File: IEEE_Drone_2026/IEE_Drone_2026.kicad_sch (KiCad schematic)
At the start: 31 parts, among them IC1 TPSM84209RKHT, IC2 TPSM84209RKHT, J1 ESC, J10 M2, J11 Conn_01x02_Socket, J2 M4 Mounting, J3 M4 Mounting, J4 M4 Mounting, J5 M4 Mounting, J6 Pixy2, J7 M2, J8 M2, J9 M2, Q1 2N2222, U1 MS560702BA03-50

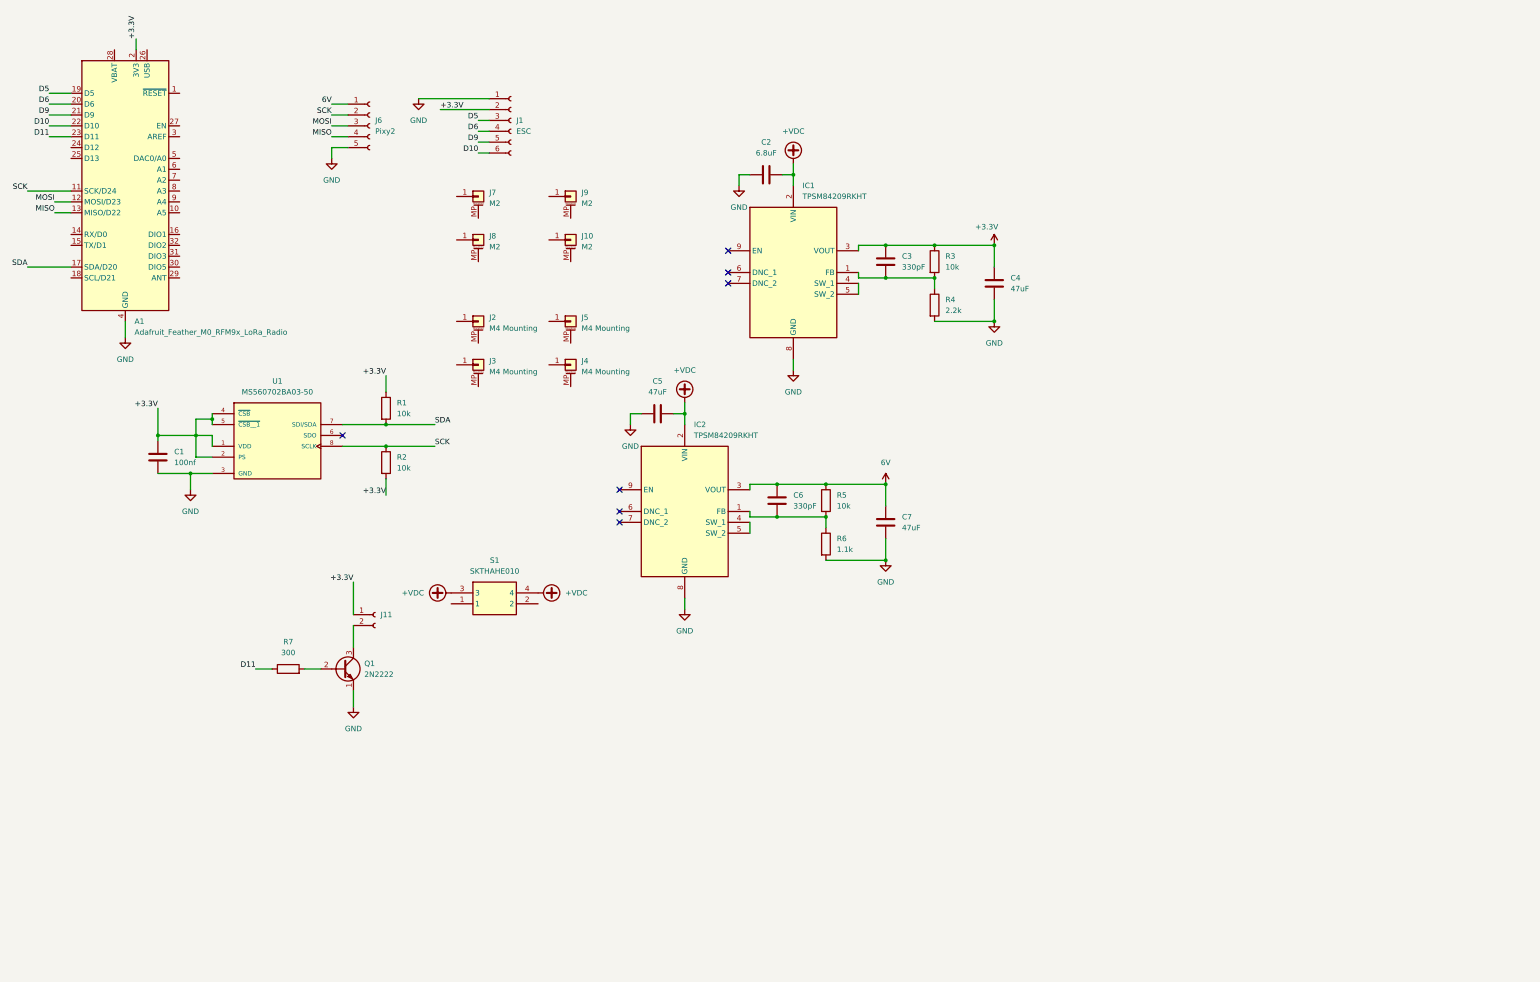
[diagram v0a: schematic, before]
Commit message: update sch last time before redesign
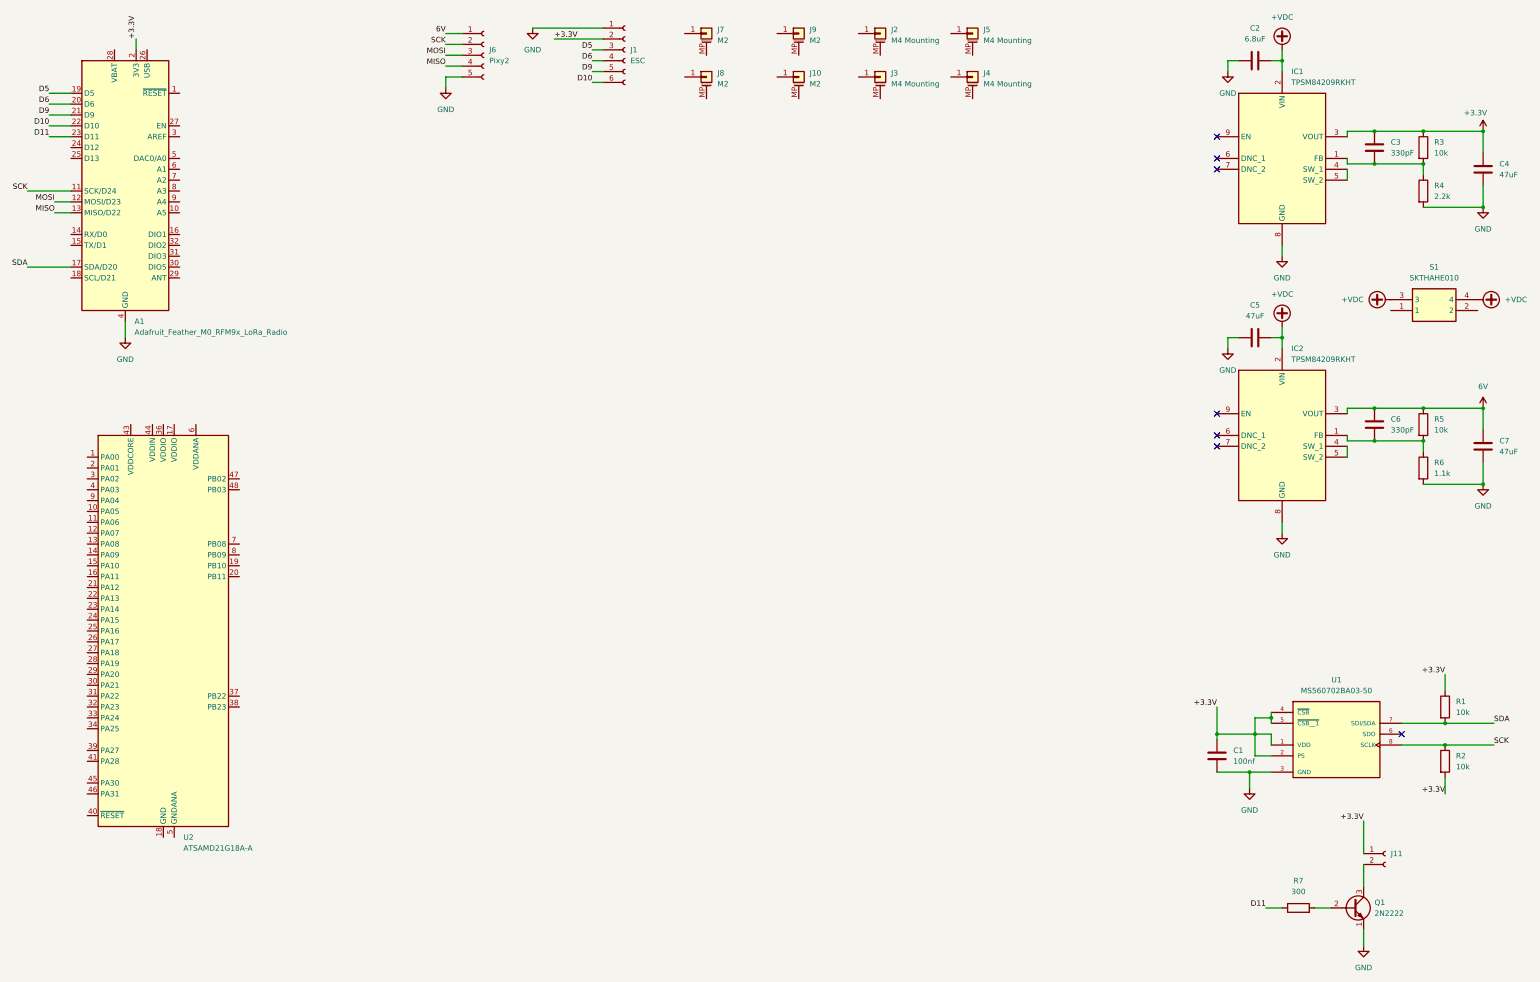
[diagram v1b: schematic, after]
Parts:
- added U2: ATSAMD21G18A-A, Package_QFP:TQFP-48_7x7mm_P0.5mm, symbol MCU_Microchip_SAMD:ATSAMD21G18A-A
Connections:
- new net: U2.18 (GND), U2.35 (GND), U2.42 (GND)
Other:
- moved on the sheet: C1, C2, C3, C4, C5, C6, C7, IC1, IC2, J1, J10, J11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
